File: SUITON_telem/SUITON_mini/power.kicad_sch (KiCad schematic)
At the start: 32 parts, among them J1 Conn_01x02_Pin, Q2 AO3407A, Q5 BSS138, U2 TPS63070RNMR, U3 TPS2121RUXR, U4 AP2112K-3.3TRG1

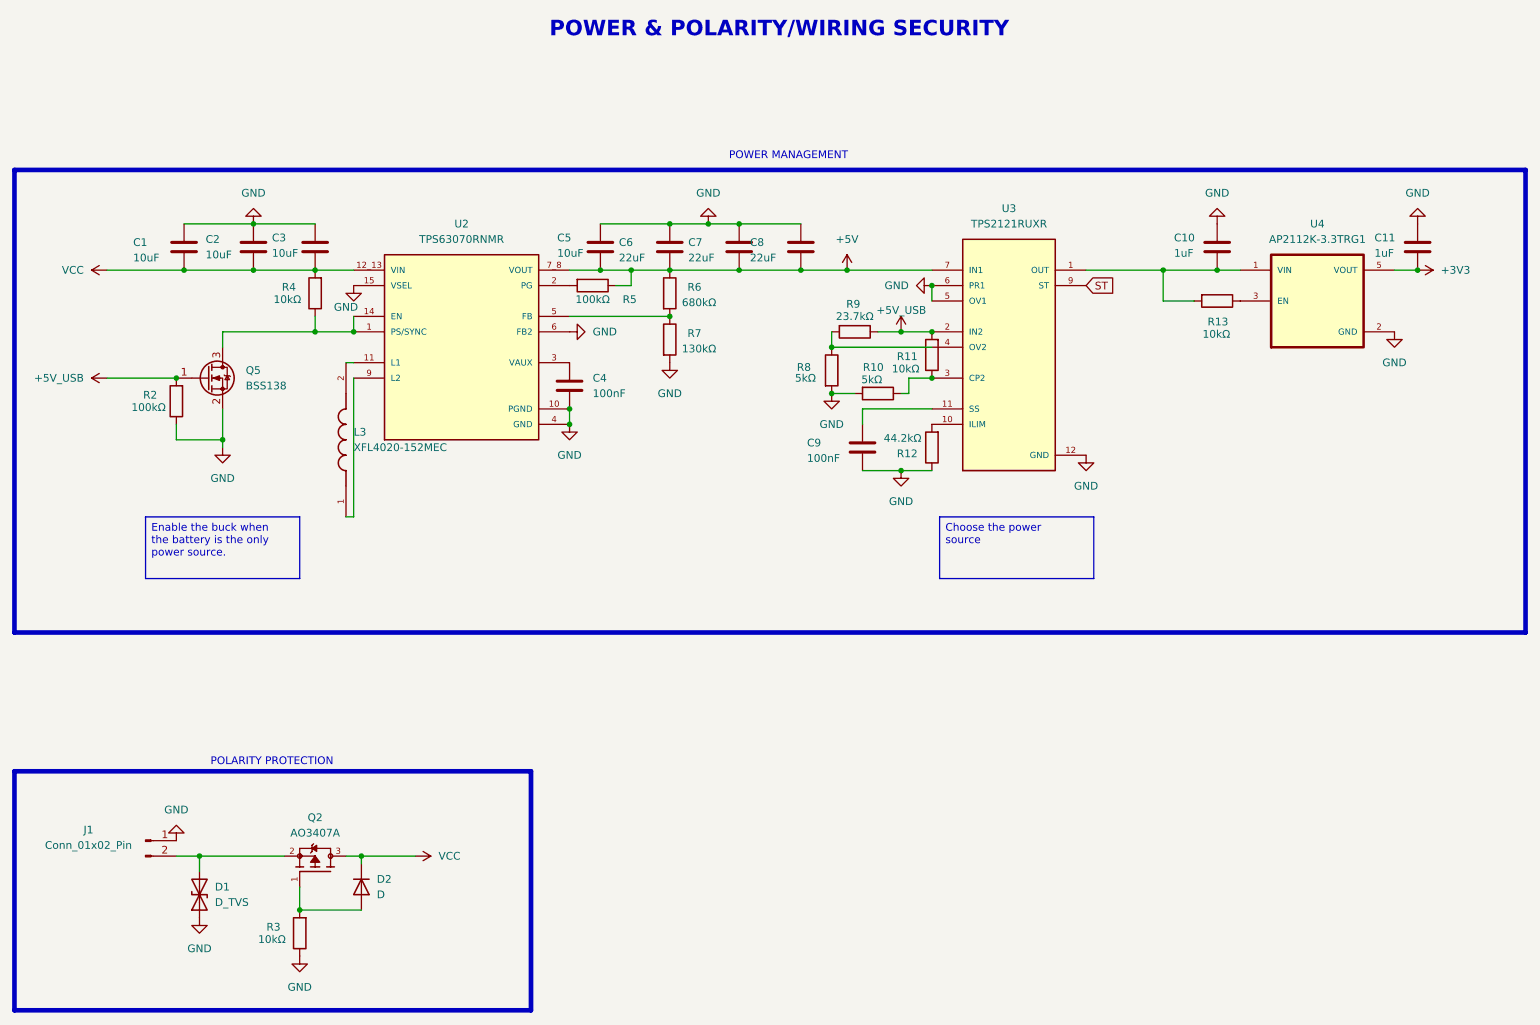
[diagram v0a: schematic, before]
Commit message: Premier placement global
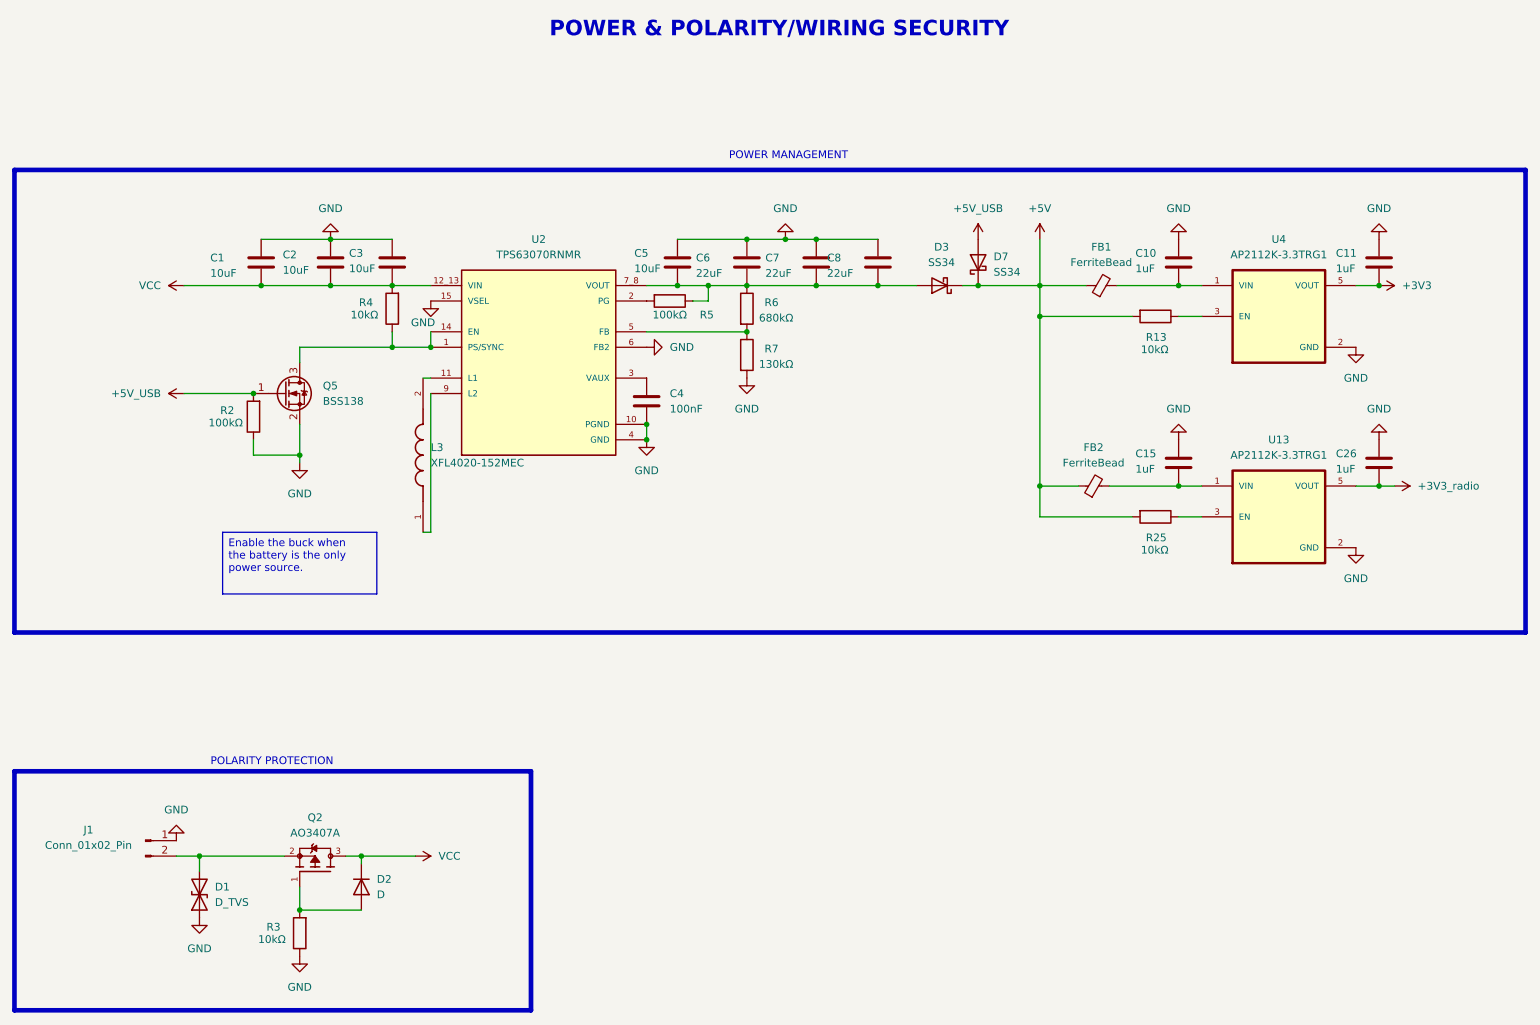
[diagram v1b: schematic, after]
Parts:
- removed C9: 100nF, Capacitor_SMD:C_0603_1608Metric, symbol Device:C
- removed R10, R8: 5kΩ, symbol Device:R
- removed R11: 10kΩ, symbol Device:R
- removed R12: 44.2kΩ, symbol Device:R
- removed R9: 23.7kΩ, symbol Device:R
- removed U3: TPS2121RUXR, TPS2121RUXR:IC_TPS2121RUXR, symbol TPS2121RUXR:TPS2121RUXR
- added C15, C26: 1uF, Capacitor_SMD:C_0603_1608Metric_Pad1.08x0.95mm_HandSolder, symbol Device:C
- added D3, D7: SS34, Diode_SMD:D_SMA, symbol Diode:SS34
- added FB1, FB2: FerriteBead, Inductor_SMD:L_0805_2012Metric, symbol Device:FerriteBead_Small
- added R25: 10kΩ, symbol Device:R
- added U13: AP2112K-3.3TRG1, AP2112K-3.3TRG1 (1):SOT95P285X140-5N, symbol AP2112K-3.3TRG1:AP2112K-3.3TRG1
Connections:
- net +5V: now also R13.2, D3.1 (K), D7.1 (K), FB1.1, FB2.1, R25.2; no longer C5.1, C6.1, C7.1, C8.1, R5.1, R6.1, U2.7_8 (VOUT)
- net +5V_USB: now also D7.2 (A)
- net GND: now also C15.2, C26.2, U13.2 (GND)
- net at C10.1, U4.1 (VIN): now also FB1.2; no longer R13.2
- new net: C5.1, C6.1, C7.1, C8.1, D3.2 (A), R5.1, R6.1, U2.7_8 (VOUT)
- new net: C15.1, FB2.2, U13.1 (VIN)
- new net: R25.1, U13.3 (EN)
- new net +3V3_radio: C26.1, U13.5 (VOUT)
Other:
- moved on the sheet: C1, C10, C11, C2, C3, C4, C5, C6, C7, C8, L3, Q5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

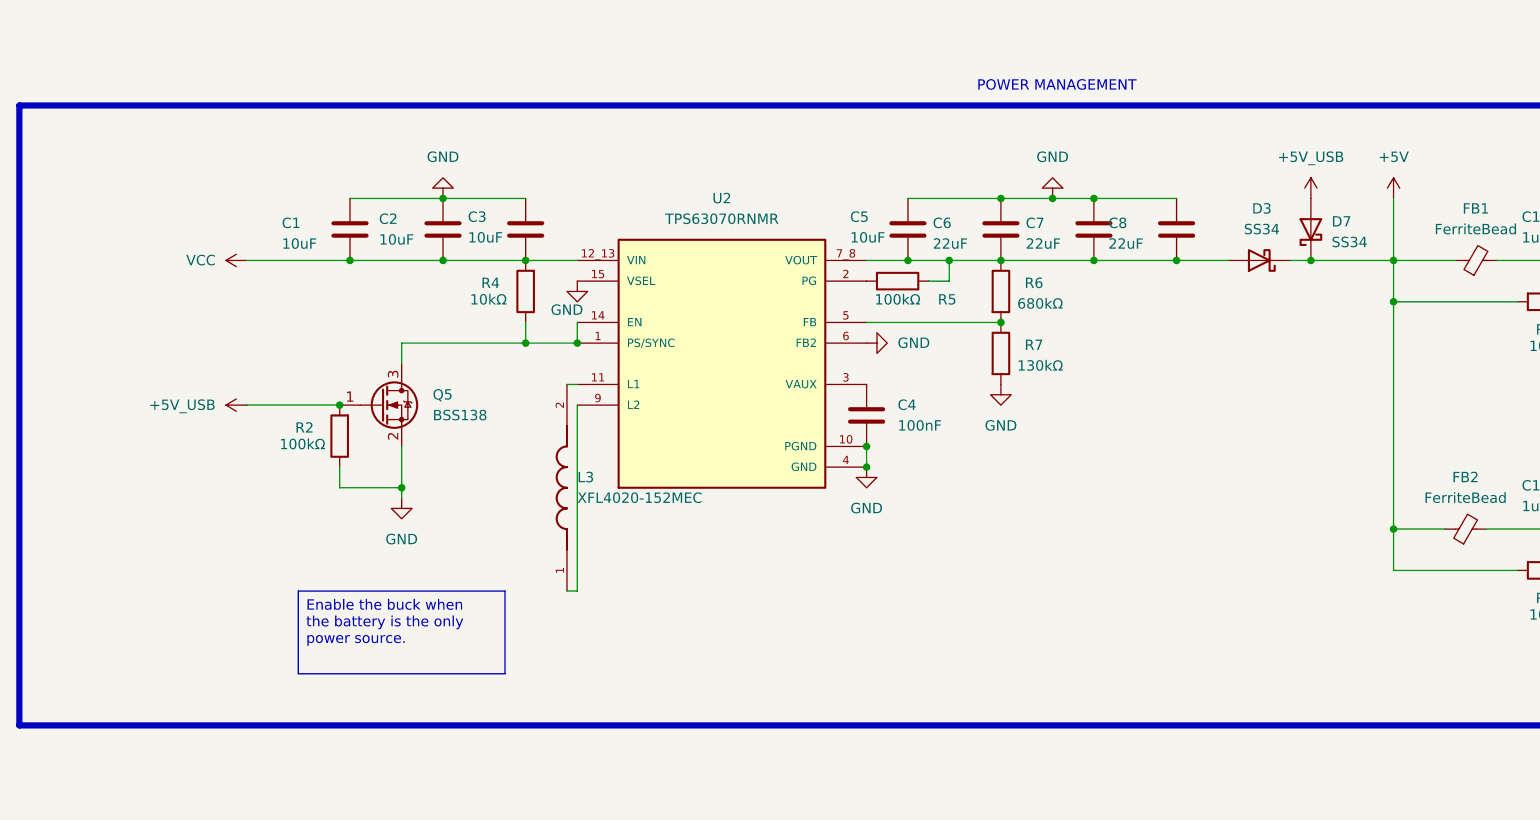
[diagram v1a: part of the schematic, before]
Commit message: Shape
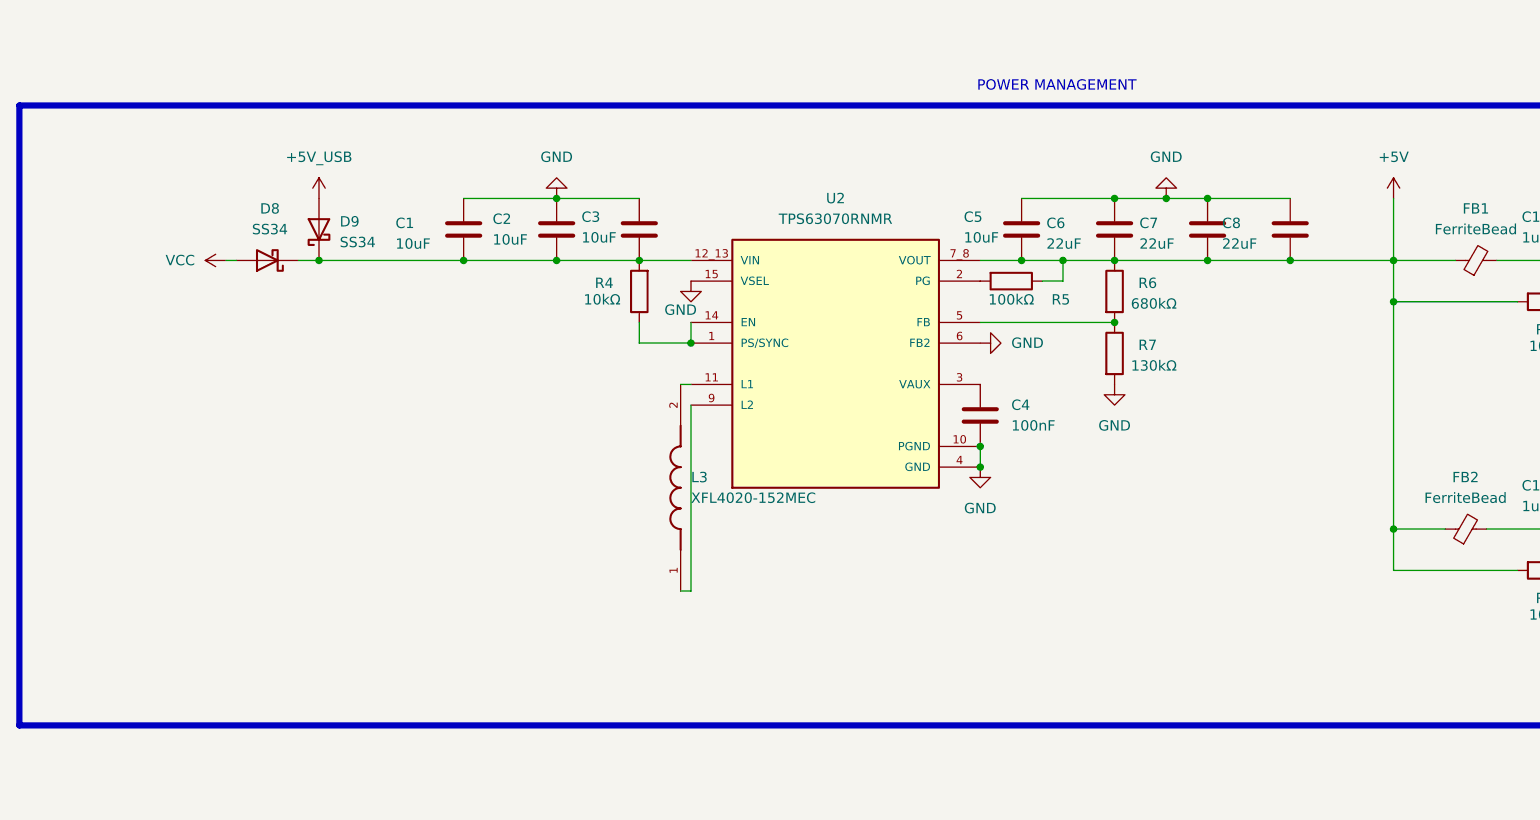
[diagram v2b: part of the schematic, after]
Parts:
- removed D3, D7: SS34, Diode_SMD:D_SMA, symbol Diode:SS34
- removed Q5: BSS138, Package_TO_SOT_SMD:SOT-23, symbol Transistor_FET:BSS138
- removed R2: 100kΩ, Resistor_SMD:R_0402_1005Metric, symbol Device:R
- added D8, D9: SS34, Diode_SMD:D_SMA, symbol Diode:SS34
- J1: footprint (none) -> TerminalBlock_Phoenix:TerminalBlock_Phoenix_MPT-0,5-2-2.54_1x02_P2.54mm_Horizontal
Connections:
- net +5V: now also C5.1, C6.1, C7.1, C8.1, R5.1, R6.1, U2.7_8 (VOUT)
- net +5V_USB: now also D9.2 (A)
- net VCC: now also D8.2 (A); no longer C1.1, C2.1, C3.1, R4.2, U2.12_13 (VIN)
- new net: C1.1, C2.1, C3.1, D8.1 (K), D9.1 (K), R4.2, U2.12_13 (VIN)
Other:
- moved on the sheet: C1, C2, C3, C4, C5, C6, C7, C8, L3, R4, R5, R6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

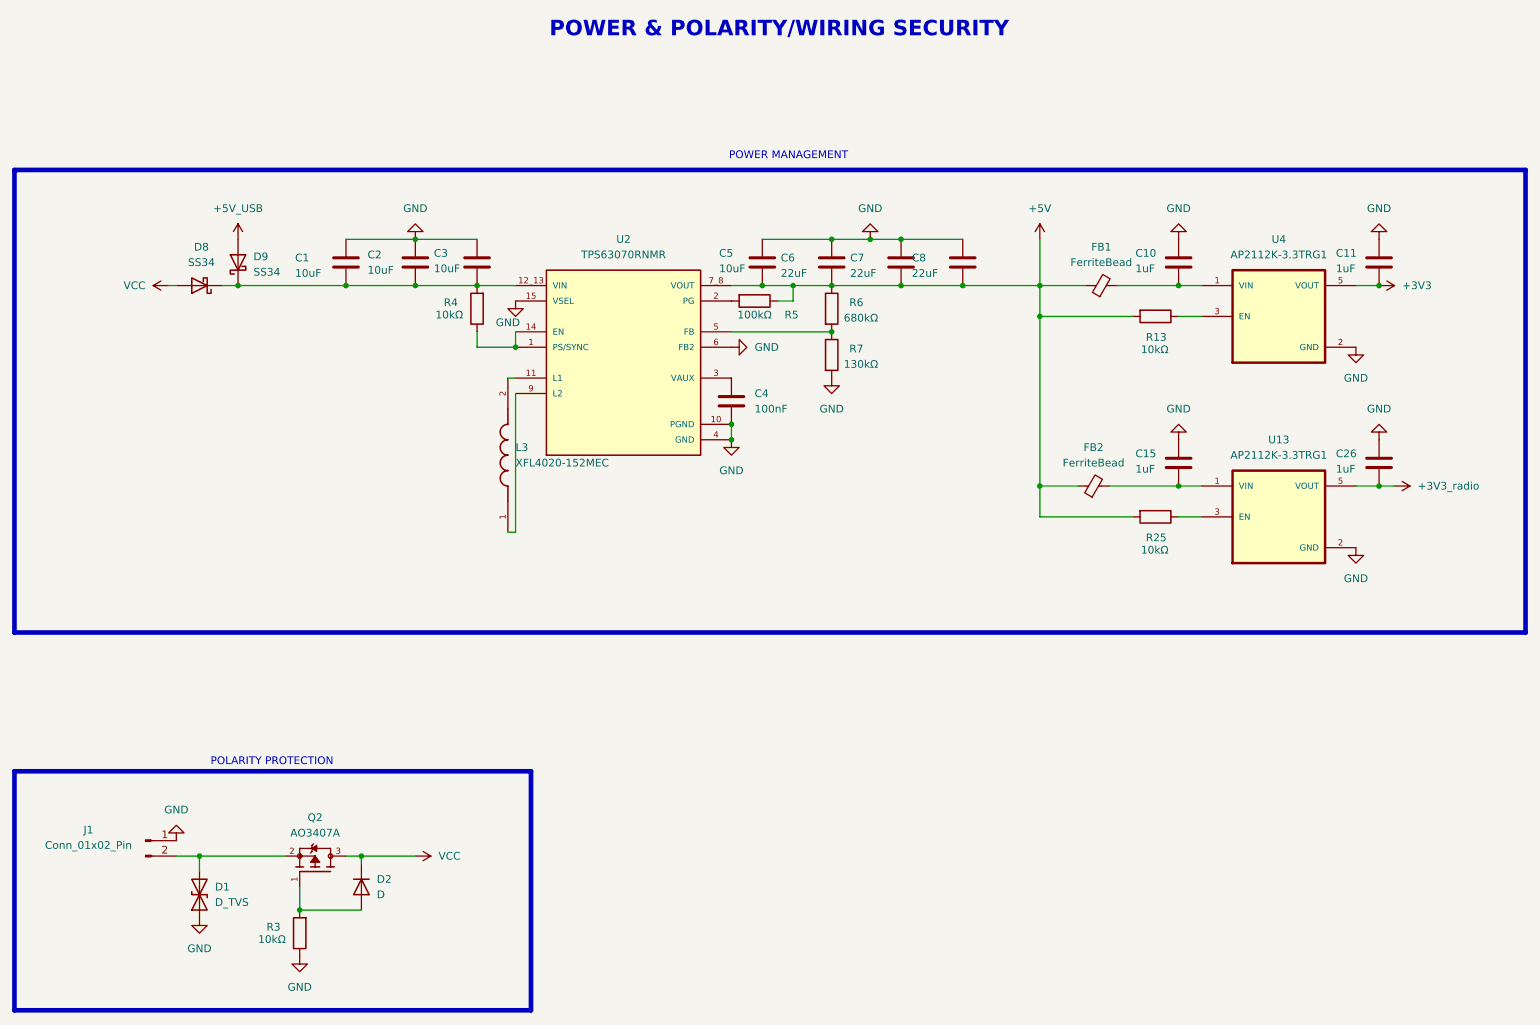
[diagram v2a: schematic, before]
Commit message: Suiton mini
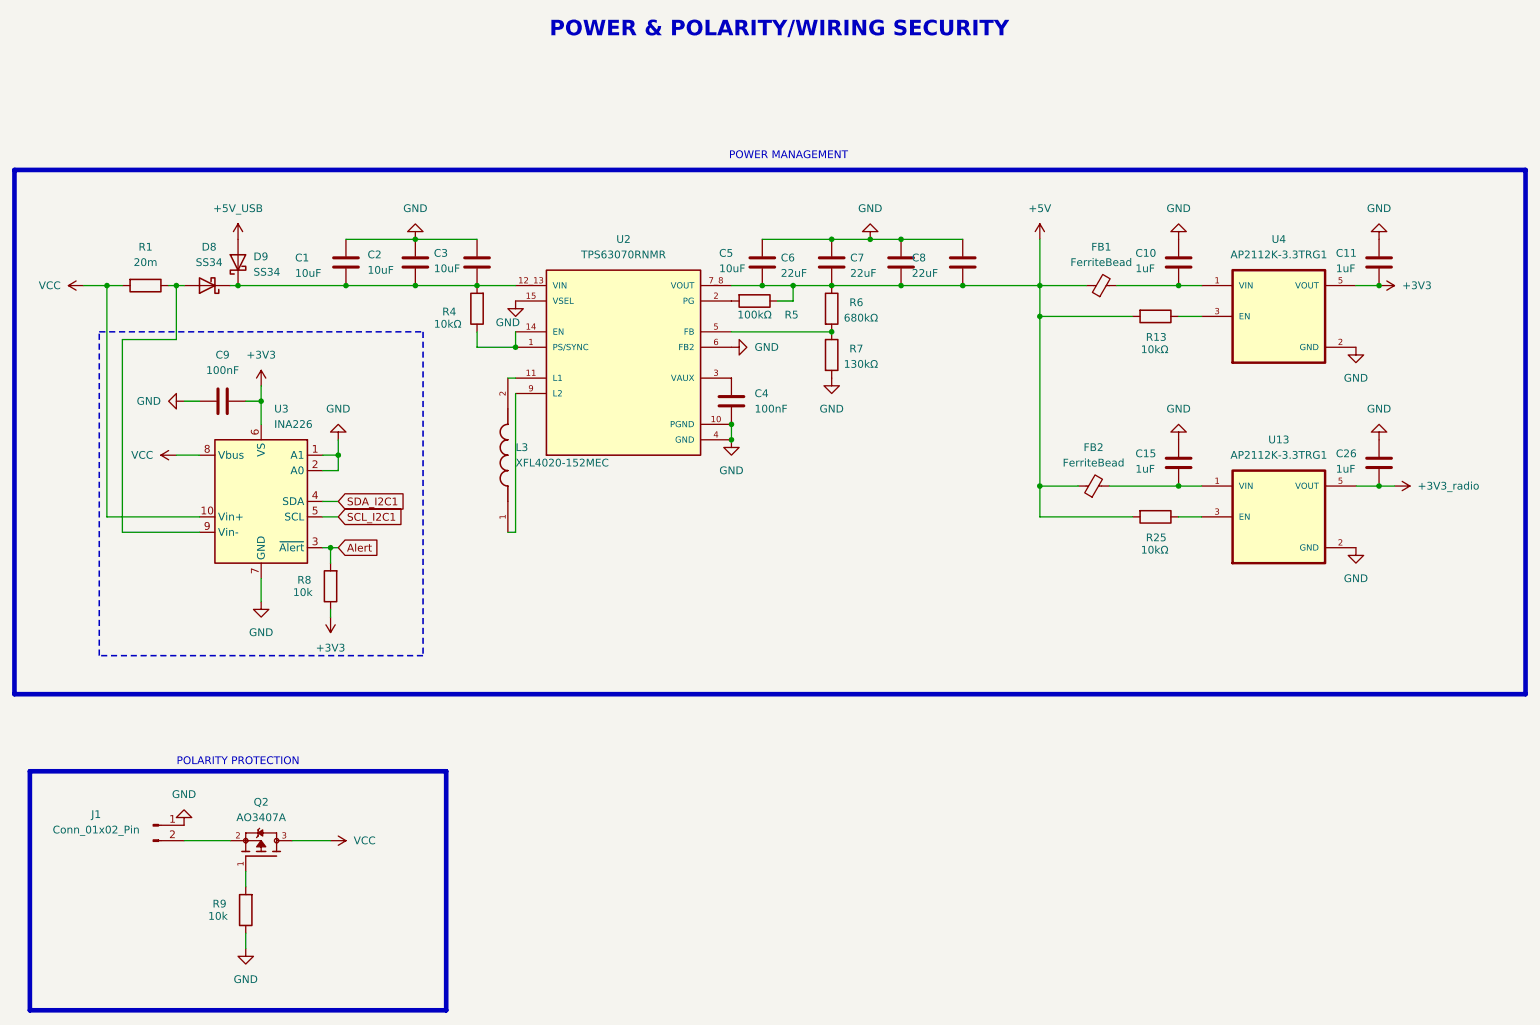
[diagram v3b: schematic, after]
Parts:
- removed D1: D_TVS, symbol Device:D_TVS
- removed D2: D, symbol Device:D
- removed R3: 10kΩ, symbol Device:R
- added C9: 100nF, Capacitor_SMD:C_0402_1005Metric, symbol Device:C
- added R1: 20m, Resistor_SMD:R_1206_3216Metric, symbol Device:R
- added R8, R9: 10k, Resistor_SMD:R_0402_1005Metric, symbol Device:R
- added U3: INA226, Package_SO:TSSOP-10_3x3mm_P0.5mm, symbol Sensor_Energy:INA226
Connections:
- net +3V3: now also C9.2, R8.1, U3.6 (VS)
- net GND: now also C9.1, R9.1, U3.1 (A1), U3.2 (A0), U3.7 (GND)
- net VCC: now also R1.2, U3.10 (Vin+), U3.8 (Vbus); no longer D8.2 (A)
- net at Q2.1: now also R9.2
- new net: D8.2 (A), R1.1, U3.9 (Vin-)
- new net Alert: R8.2, U3.3 (~{Alert})
- new net SCL_I2C1: U3.5 (SCL)
- new net SDA_I2C1: U3.4 (SDA)
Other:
- moved on the sheet: D8, J1, Q2
